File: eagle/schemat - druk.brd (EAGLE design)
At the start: 210 parts, among them IC1 MEGA8-AI, IC2 MEGA8-AI, IC3 MEGA8-AI, IC4 MEGA8-AI, IC5 MEGA8-AI, IC6 MEGA8-AI, Q1 N-MOSFET BSS138, Q10 N-MOSFET BSS138, Q11 N-MOSFET BSS138, Q12 N-MOSFET BSS138, Q2 N-MOSFET BSS138, Q3 N-MOSFET BSS138, Q4 N-MOSFET BSS138, Q5 N-MOSFET BSS138, Q6 N-MOSFET BSS138, Q7 N-MOSFET BSS138, Q8 N-MOSFET BSS138, Q9 N-MOSFET BSS138, U1 LCD-16X2SILK, U2 LCD-16X2SILK, U3 LCD-16X2SILK, U4 LCD-16X2SILK, U5 LCD-16X2SILK, U6 LCD-16X2SILK, Y1 16MHz, Y2 16MHz, Y3 16MHz, Y4 16MHz, Y5 16MHz, Y6 16MHz

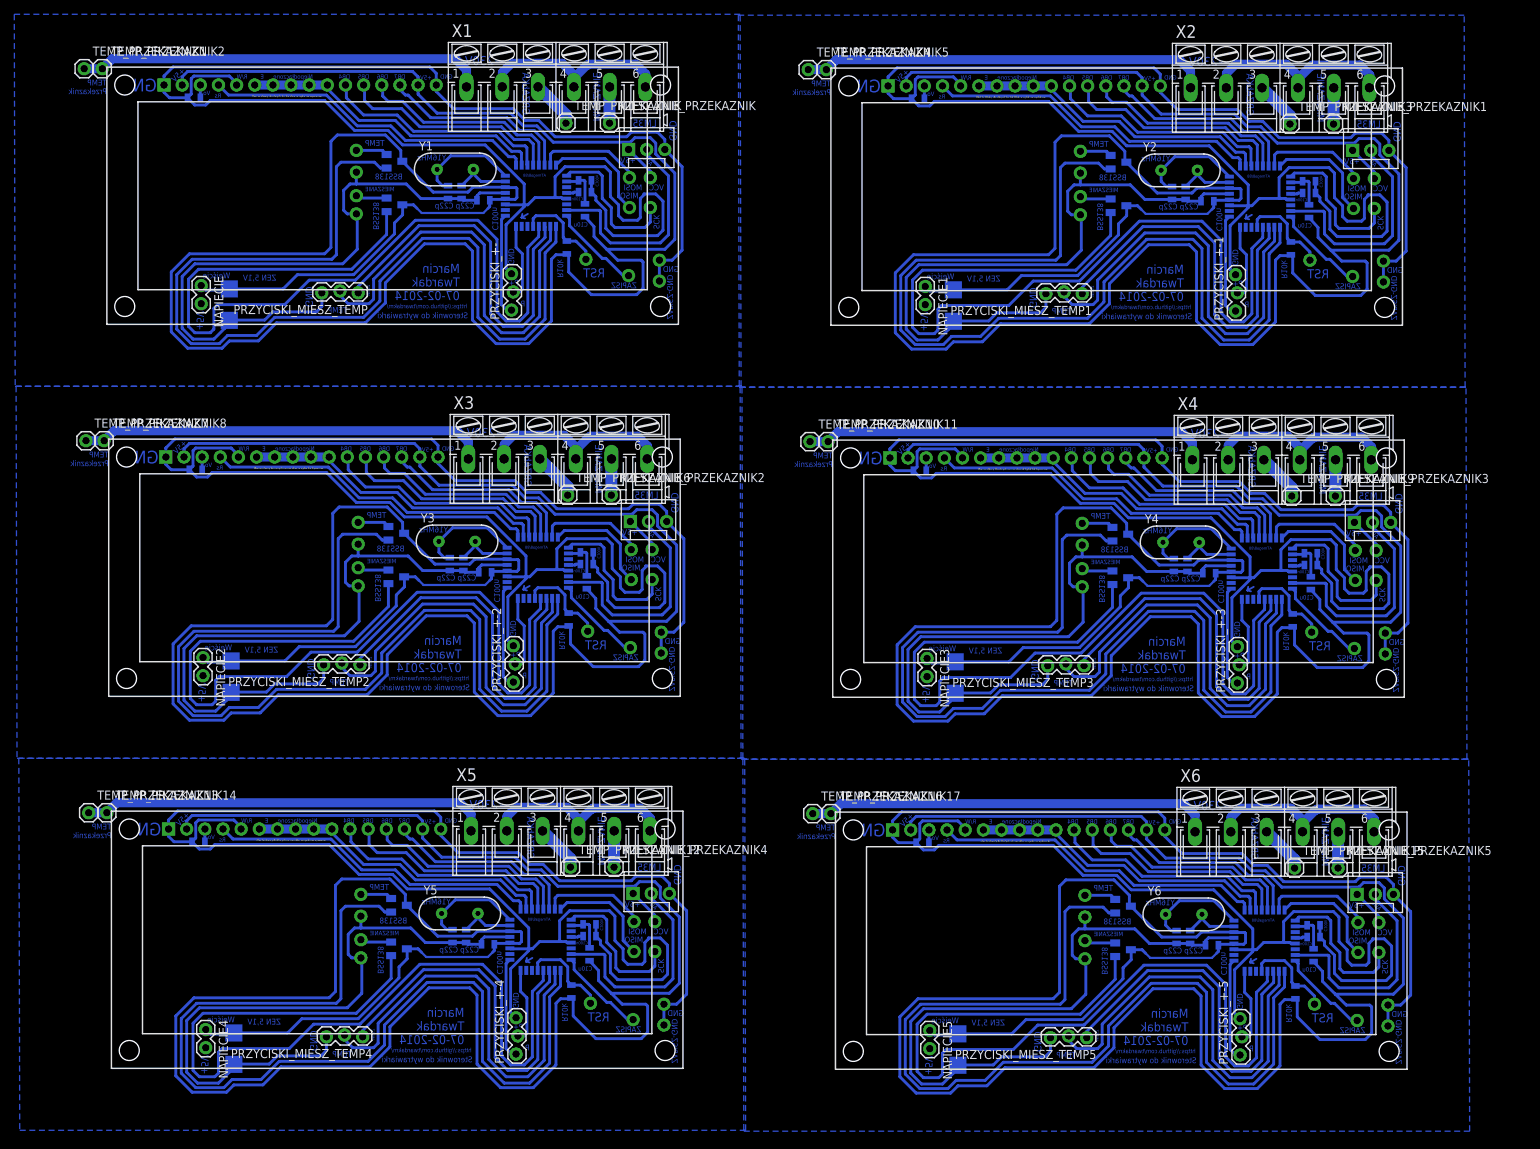
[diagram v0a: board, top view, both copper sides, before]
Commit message: kolejne poprawki
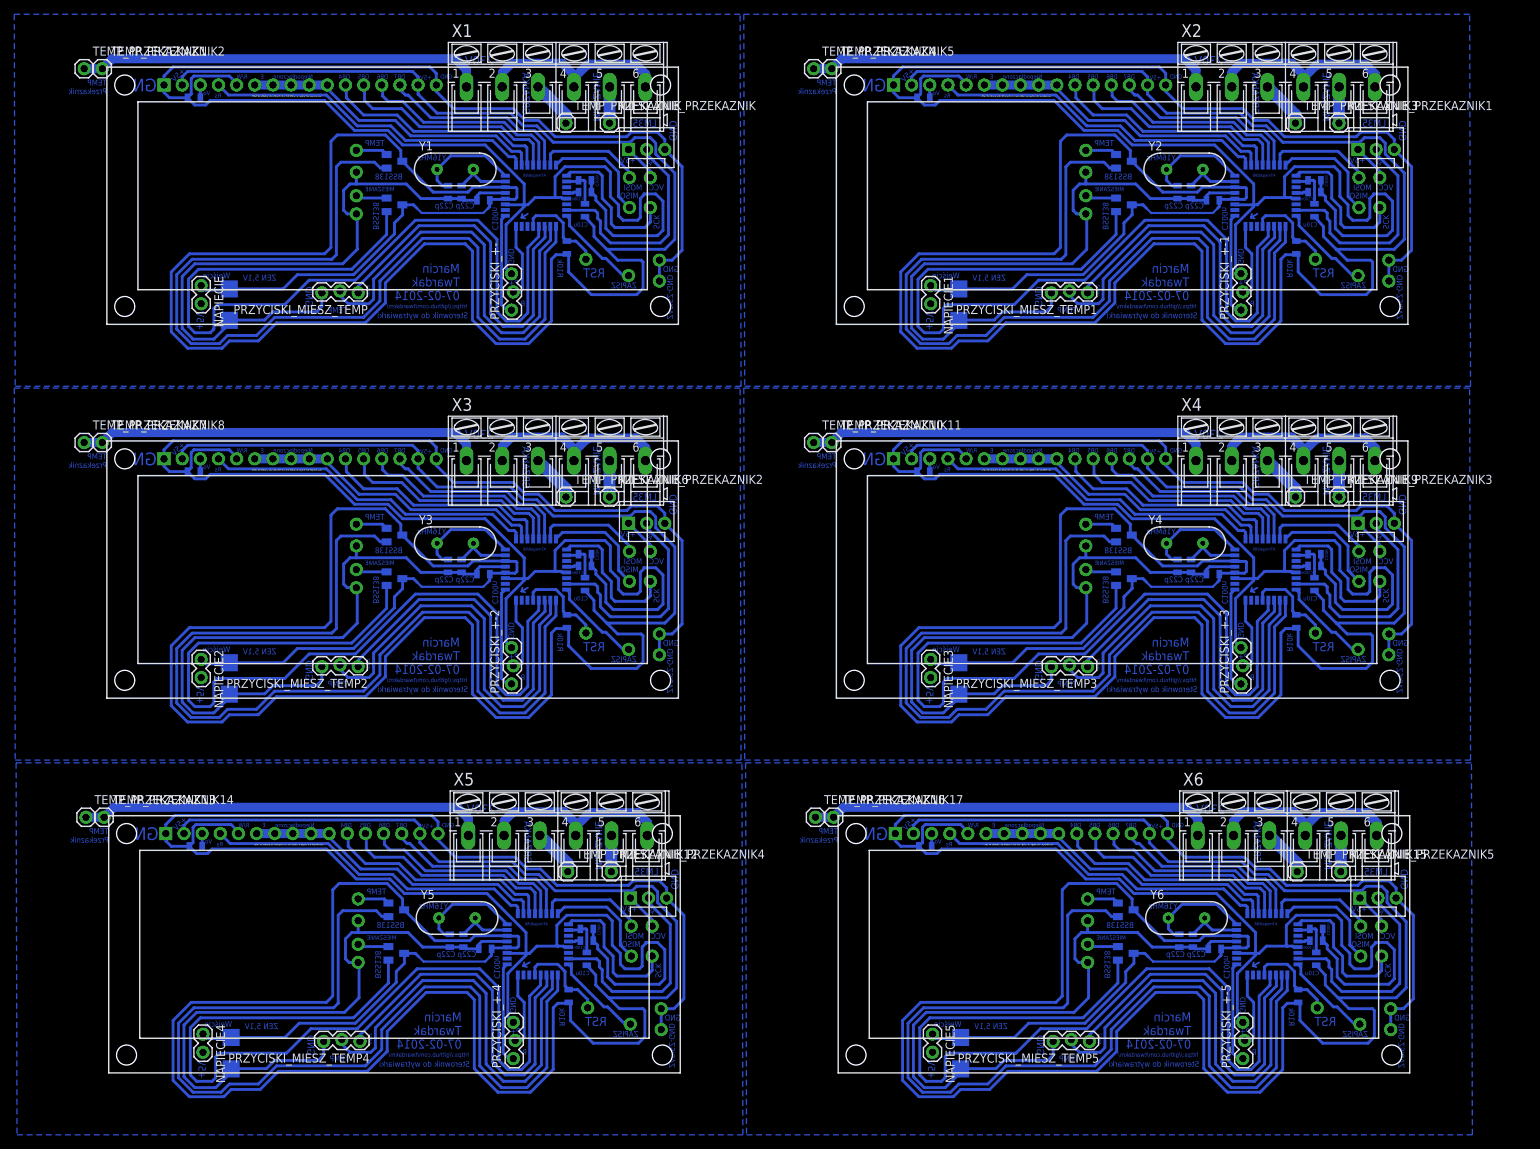
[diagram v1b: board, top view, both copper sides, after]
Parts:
- moved IC2 0.77 mm to (167.9, 80.0)
- moved MIESZANIE1 0.77 mm to (142.7, 80.0)
- moved RESET1 0.77 mm to (174.9, 71.1)
- moved TEMP_PRZEKAZNIK4 0.77 mm to (104.6, 97.8)
- moved TEMP_PRZEKAZNIK5 0.77 mm to (107.2, 97.8)
- moved U2 0.77 mm to (147.8, 80.0)
- moved ZAPISZ1 0.77 mm to (180.8, 68.8)
- moved ZAPISZ_GND1 0.77 mm to (185.2, 68.1)
- moved C10 0.77 mm to (160.5, 79.4)
- moved C6 0.77 mm to (174.8, 80.5)
- moved C7 0.77 mm to (174.8, 82.2)
- moved C8 0.77 mm to (157.5, 80.5)
- moved C9 0.77 mm to (155.6, 80.5)
- moved GND1 0.77 mm to (185.2, 71.0)
- moved L2 0.77 mm to (174.8, 78.0)
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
